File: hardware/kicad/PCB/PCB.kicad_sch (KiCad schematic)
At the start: 19 parts, among them J1 USB_C_Receptacle_PowerOnly_6P, J2 Conn_01x05_Socket, J3 Conn_01x02, U1 STM32G030F6Px, U2 MCP73831-2-OT, U3 DW01A, U4 FS8205A_C2830320

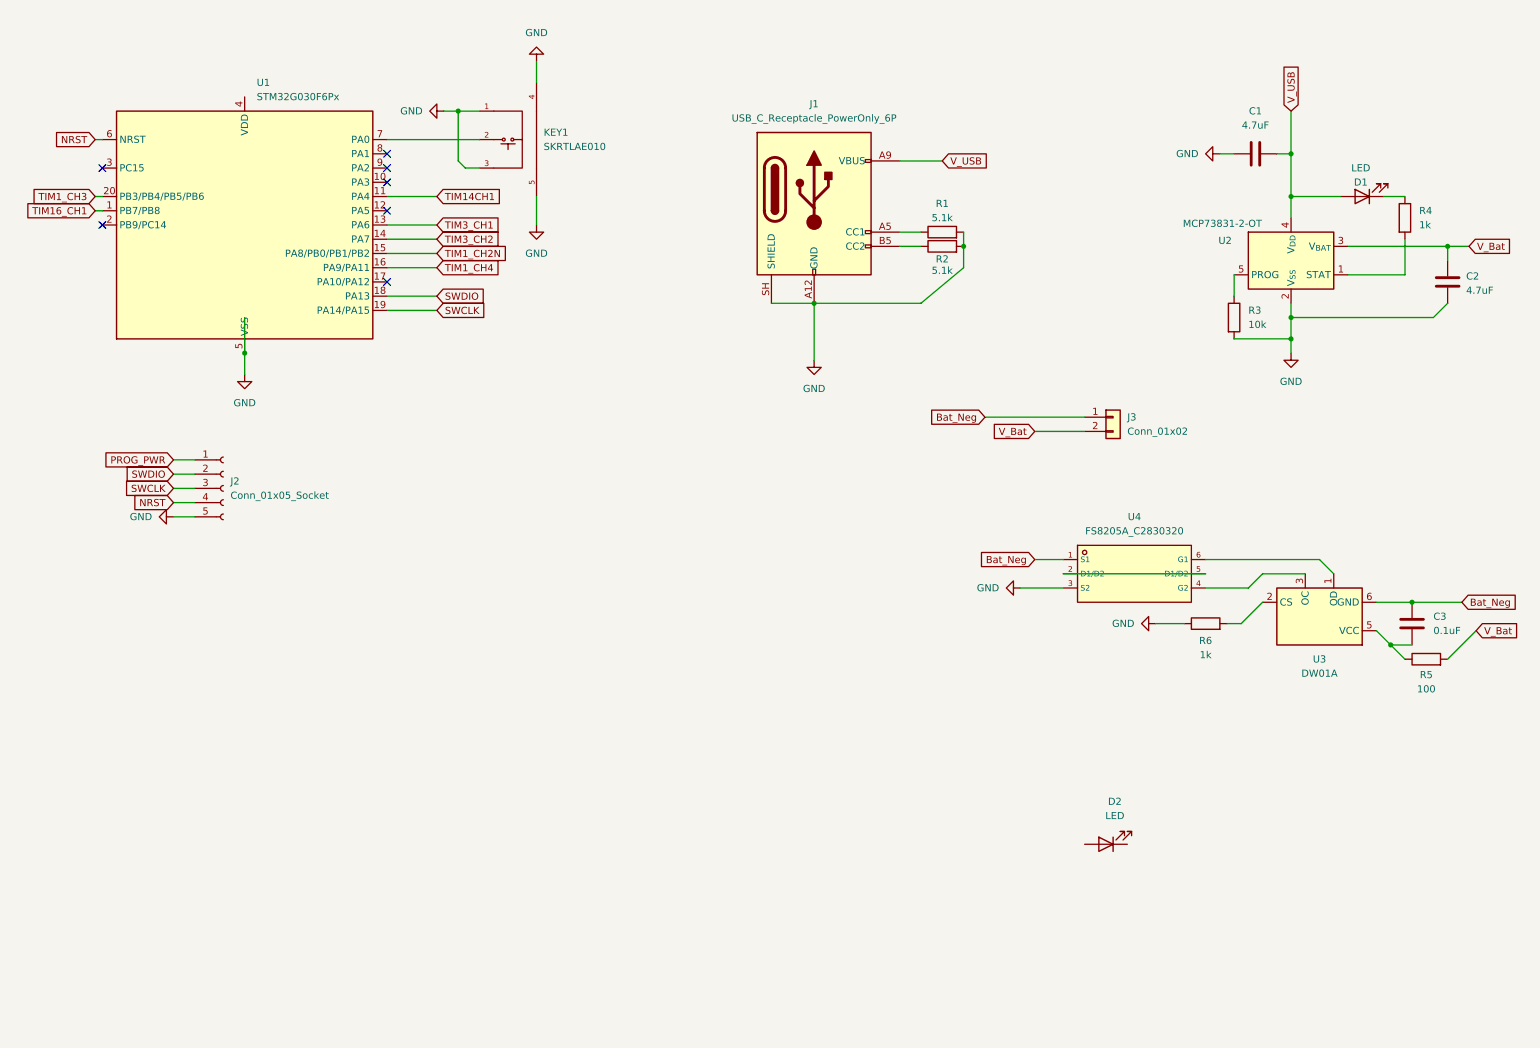
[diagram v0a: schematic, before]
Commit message: updated PCB design
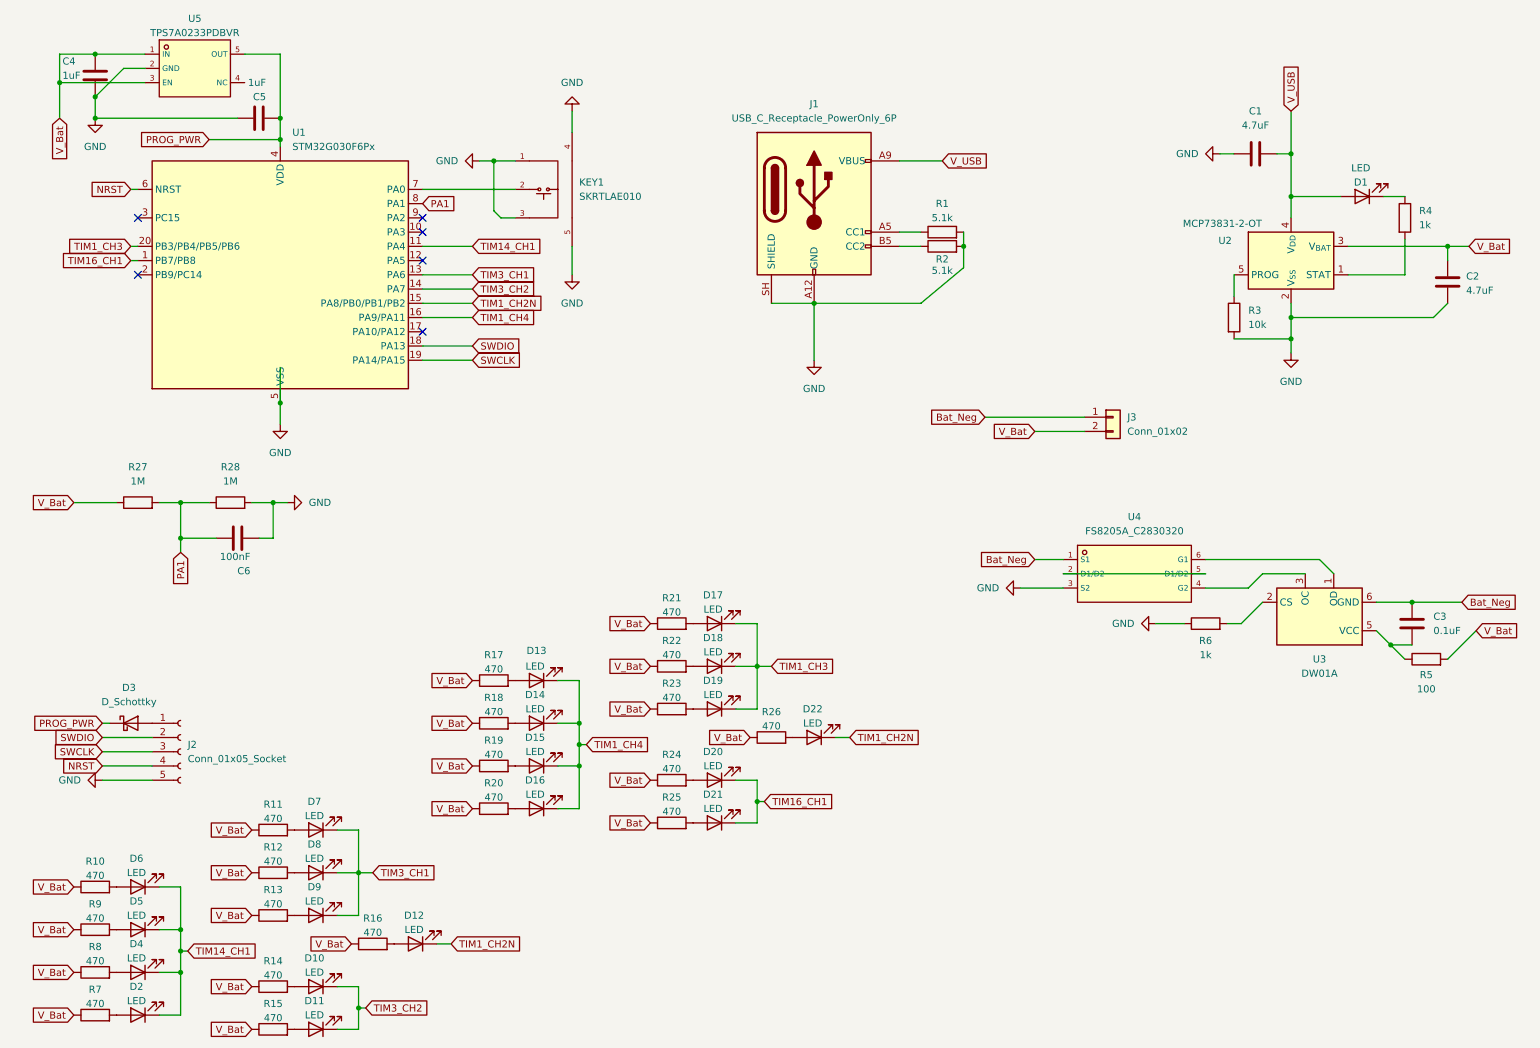
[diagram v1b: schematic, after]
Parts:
- added C4, C5: 1uF, Capacitor_SMD:C_0603_1608Metric, symbol Device:C
- added C6: 100nF, Capacitor_SMD:C_0603_1608Metric, symbol Device:C
- added D10, D11, D12, D13, D14, D15, D16, D17, D18, D19, D20, D21, D22, D4, D5, D6, D7, D8, D9: LED, Diode_SMD:D_0603_1608Metric, symbol Device:LED
- added D3: D_Schottky, Sensor_Humidity:Sensirion_DFN-4_1.5x1.5mm_P0.8mm_SHT4x_NoCentralPad, symbol Device:D_Schottky
- added R10, R11, R12, R13, R14, R15, R16, R17, R18, R19, R20, R21, R22, R23, R24, R25, R26, R7, R8, R9: 470, Resistor_SMD:R_0603_1608Metric, symbol Device:R
- added R27, R28: 1M, Resistor_SMD:R_0603_1608Metric, symbol Device:R
- added U5: TPS7A0233PDBVR, JLC2KiCad:SOT-23-5_L2.9-W1.6-P0.95-LS2.8-BR, symbol JLC2KiCad2:TPS7A0233PDBVR
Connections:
- net TIM14CH1 is gone; now on net TIM14_CH1: U1.11 (PA4)
- net GND: now also C4.2, C5.1, C6.2, R28.2, U5.2 (GND)
- net PROG_PWR: now also U1.4 (VDD), C5.2, D3.1 (K), U5.5 (OUT); no longer J2.1 (Pin_1)
- net TIM16_CH1: now also D20.1 (K), D21.1 (K)
- net TIM1_CH2N: now also D12.1 (K), D22.1 (K)
- net TIM1_CH3: now also D17.1 (K), D18.1 (K), D19.1 (K)
- net TIM1_CH4: now also D13.1 (K), D14.1 (K), D15.1 (K), D16.1 (K)
- net TIM3_CH1: now also D7.1 (K), D8.1 (K), D9.1 (K)
- net TIM3_CH2: now also D10.1 (K), D11.1 (K)
- net V_Bat: now also C4.1, R10.1, R11.1, R12.1, R13.1, R14.1, R15.1, R16.1, R17.1, R18.1, R19.1, R20.1, R21.1, R22.1, R23.1, R24.1, R25.1, R26.1, R27.1, R7.1, R8.1, R9.1, U5.1 (IN), U5.3 (EN)
- net TIM14_CH1: now reaches D2.1 (K)
- net TIM14_CH1: now also D4.1 (K), D5.1 (K), D6.1 (K)
- net at D2.2 (A): now also R7.2
- net PA1: now reaches U1.8 (PA1)
- net PA1: now also C6.1, R27.2, R28.1
- new net: D22.2 (A), R26.2
- new net: D18.2 (A), R22.2
- new net: D4.2 (A), R8.2
- new net: D17.2 (A), R21.2
- new net: D11.2 (A), R15.2
- new net: D7.2 (A), R11.2
- new net: D16.2 (A), R20.2
- new net: D21.2 (A), R25.2
- new net: D15.2 (A), R19.2
- new net: D8.2 (A), R12.2
- new net: D9.2 (A), R13.2
- new net: D6.2 (A), R10.2
- new net: D19.2 (A), R23.2
- new net: D14.2 (A), R18.2
- new net: D20.2 (A), R24.2
- new net: D3.2 (A), J2.1 (Pin_1)
- new net: D12.2 (A), R16.2
- new net: D5.2 (A), R9.2
- new net: D10.2 (A), R14.2
- new net: D13.2 (A), R17.2
- no-connect marks 7 -> 6
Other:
- moved on the sheet: D2, J2, KEY1, U1
